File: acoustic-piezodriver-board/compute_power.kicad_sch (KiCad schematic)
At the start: 31 parts, among them J301 Conn_02x06_Odd_Even, U10 NCE6005AS, U302 TMCS1108A3UQDR, U9 LM3478MM

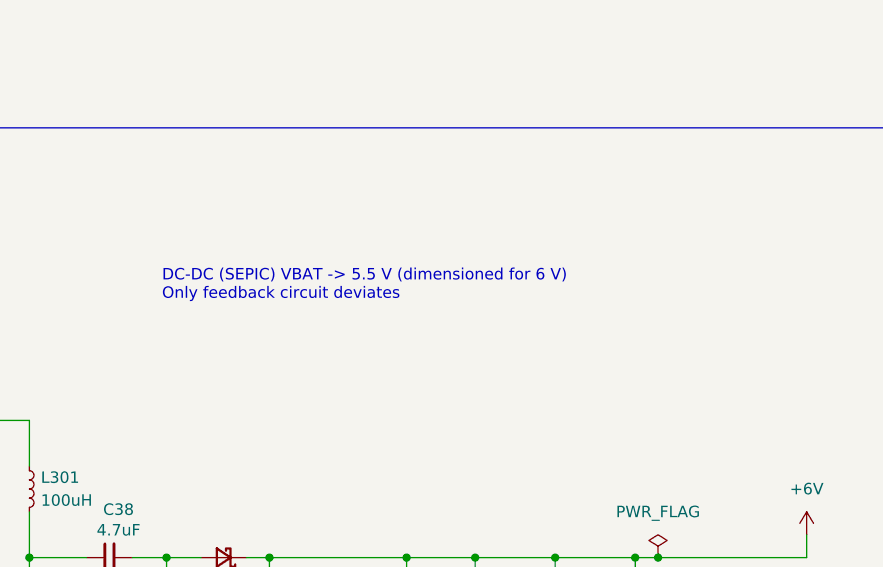
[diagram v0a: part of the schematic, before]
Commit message: added gerbers
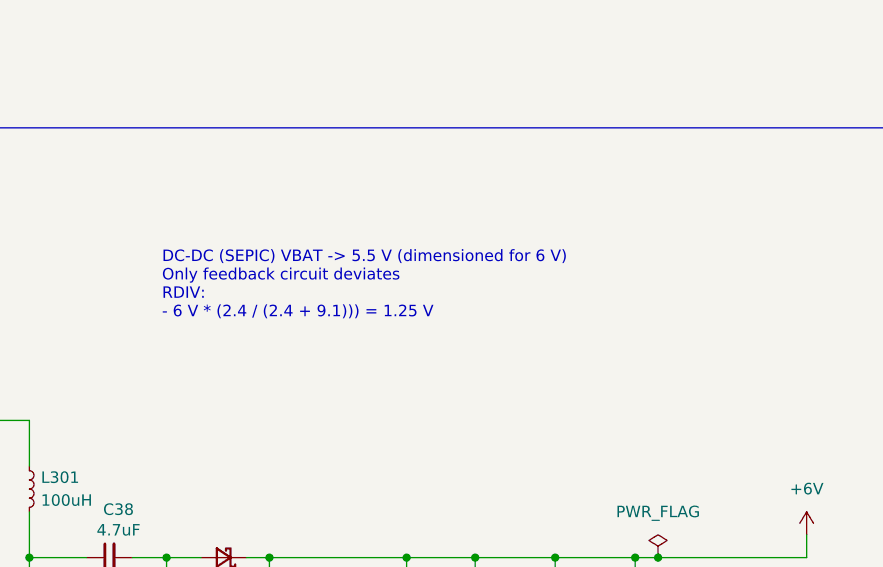
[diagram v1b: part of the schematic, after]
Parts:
- TP301, TP302: now left out of the parts list
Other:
- note added: "DC-DC (SEPIC) VBAT -> 5.5 V (dimensioned for 6 V) Only feedback circuit deviates RDIV: - 6 V * (2.4 / (2.4 + 9.1))) = 1.25 V"
- note removed: "DC-DC (SEPIC) VBAT -> 5.5 V (dimensioned for 6 V) Only feedback circuit deviates"
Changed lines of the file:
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@@
 		)
 	)
-	(text "DC-DC (SEPIC) VBAT -> 5.5 V (dimensioned for 6 V)\nOnly feedback circuit deviates"
+	(text "DC-DC (SEPIC) VBAT -> 5.5 V (dimensioned for 6 V)\nOnly feedback circuit deviates\nRDIV:\n- 6 V * (2.4 / (2.4 + 9.1))) = 1.25 V"
 		(exclude_from_sim no)
 		(at 280.162 47.244 0)
@@
 		(unit 1)
 		(exclude_from_sim no)
-		(in_bom yes)
+		(in_bom no)
 		(on_board yes)
 		(dnp no)
@@
 		(unit 1)
 		(exclude_from_sim no)
-		(in_bom yes)
+		(in_bom no)
 		(on_board yes)
 		(dnp no)
